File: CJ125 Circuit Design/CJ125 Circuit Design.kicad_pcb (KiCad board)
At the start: 2 copper layers, 76.2 x 41.5 mm, 39 parts, among them IC1 SI2302CDS-T1-BE3, J2 STLink, J4 Conn_01x06_Pin, J5 Conn_01x06_Pin, U1 CJ125, U2 LM1117DT-5.0, U3 STM32F103CBTx, U5 ISO1050DUB

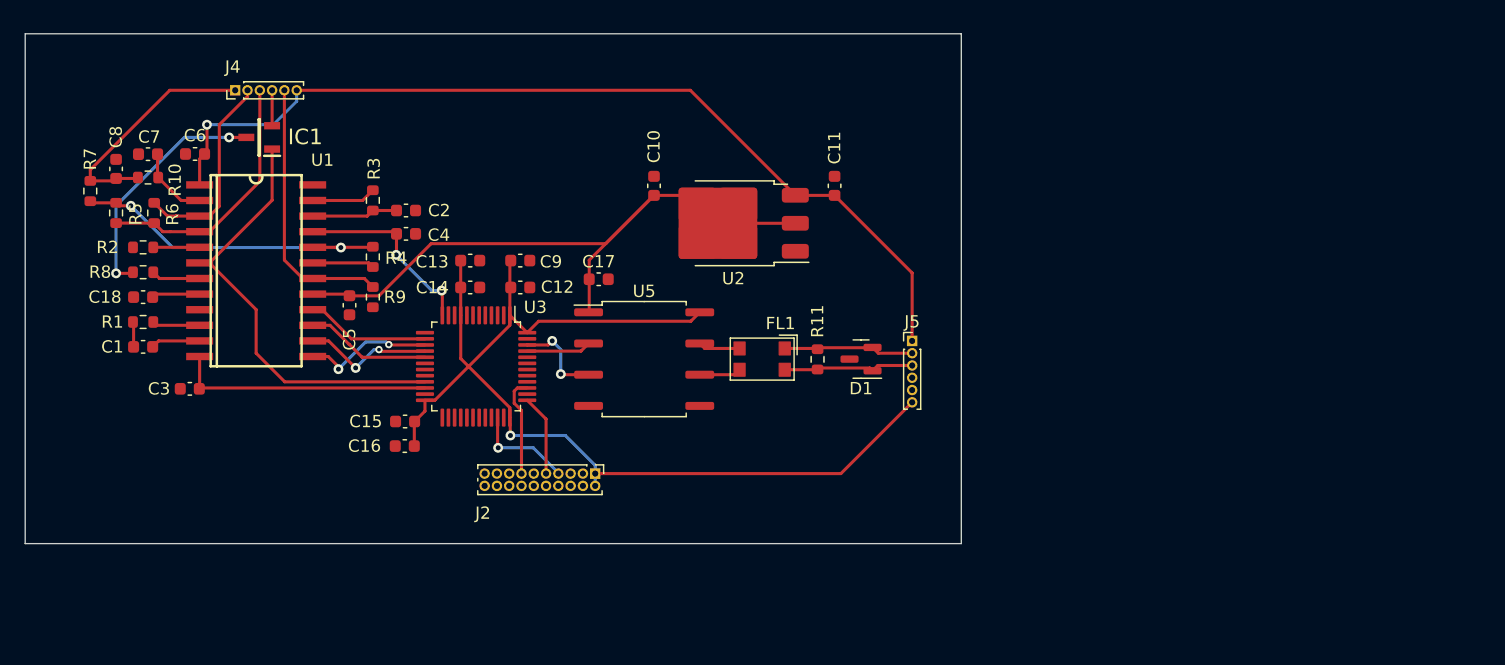
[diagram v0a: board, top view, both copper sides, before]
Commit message: new board design
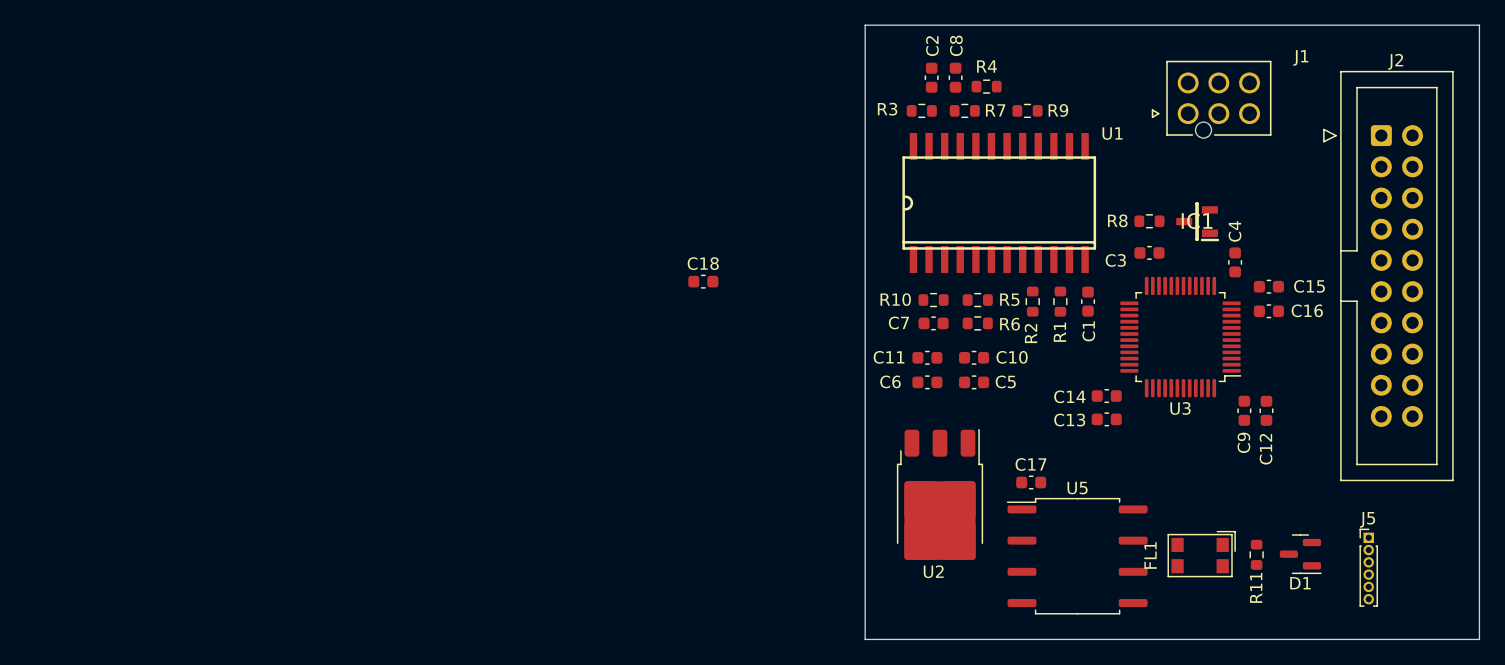
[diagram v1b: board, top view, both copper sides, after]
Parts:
- removed J4: Conn_01x06_Pin, Connector_PinHeader_1.00mm:PinHeader_1x06_P1.00mm_Vertical
- added J1: 2x3 O2 Connector, CJ125 Circuit Data:MOLEX_1053101106, F.Cu at (196.3, 57.3)
- J2: footprint Connector_PinHeader_1.00mm:PinHeader_2x10_P1.00mm_Vertical -> Connector_IDC:IDC-Header_2x10_P2.54mm_Vertical
- J5: value Conn_01x06_Pin -> 1x6 ECU Connector
- moved R8 82.0 mm to (193.1, 66.1), turned to 180 degrees
- moved C3 78.9 mm to (193.1, 68.6)
- moved C1 77.0 mm to (188.1, 72.6), turned to 90 degrees
- moved IC1 76.6 mm to (197.0, 66.1)
- moved R1 74.7 mm to (185.9, 72.6), turned to 90 degrees
- moved R2 72.5 mm to (183.6, 72.6), turned to -90 degrees
- moved R7 71.5 mm to (178.1, 57.1), turned to 180 degrees
- moved C16 71.2 mm to (202.8, 73.4), turned to 0 degrees
- moved C15 71.2 mm to (202.8, 71.4), turned to 0 degrees
- moved R5 70.5 mm to (179.1, 72.5), turned to 180 degrees
- moved J2 69.7 mm to (212.0, 59.1), turned to 0 degrees
- moved C8 68.7 mm to (177.3, 54.4)
- moved R6 67.6 mm to (179.1, 74.4), turned to 180 degrees
- moved C4 67.5 mm to (200.1, 69.4), turned to 90 degrees
- moved C7 65.4 mm to (175.5, 74.4), turned to 180 degrees
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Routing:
- net +3V3: track 89.3 -> 0.00 mm, vias 1 -> 0
- net +12V: track 75.9 -> 0.00 mm, vias 1 -> 0
- net +5V: track 55.4 -> 0.00 mm
- net /HTR_CTRL: track 35.9 -> 0.00 mm
- net Net-(U1-UP): track 27.2 -> 0.00 mm, vias 2 -> 0
- net /VM: track 21.9 -> 0.00 mm
- net /IA: track 21.1 -> 0.00 mm
- net /UR_ADC: track 21.0 -> 0.00 mm
- net Net-(IC1-D): track 19.8 -> 0.00 mm, vias 2 -> 0
- net /UN: track 19.6 -> 0.00 mm
- net /IP: track 16.4 -> 0.00 mm
- net /UA_ADC: track 15.5 -> 0.00 mm, vias 2 -> 0
- net /SPI_SCK: track 11.1 -> 0.00 mm, vias 2 -> 0
- net /SPI_MISO: track 10.7 -> 0.00 mm, vias 2 -> 0
- net /CANL: track 10.7 -> 0.00 mm
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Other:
- board size 76.2 x 41.5 mm -> 50 x 50 mm
